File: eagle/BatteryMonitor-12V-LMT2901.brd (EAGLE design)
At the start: 40.6 x 27.9 mm, 20 parts, among them IC1 LMT2901N

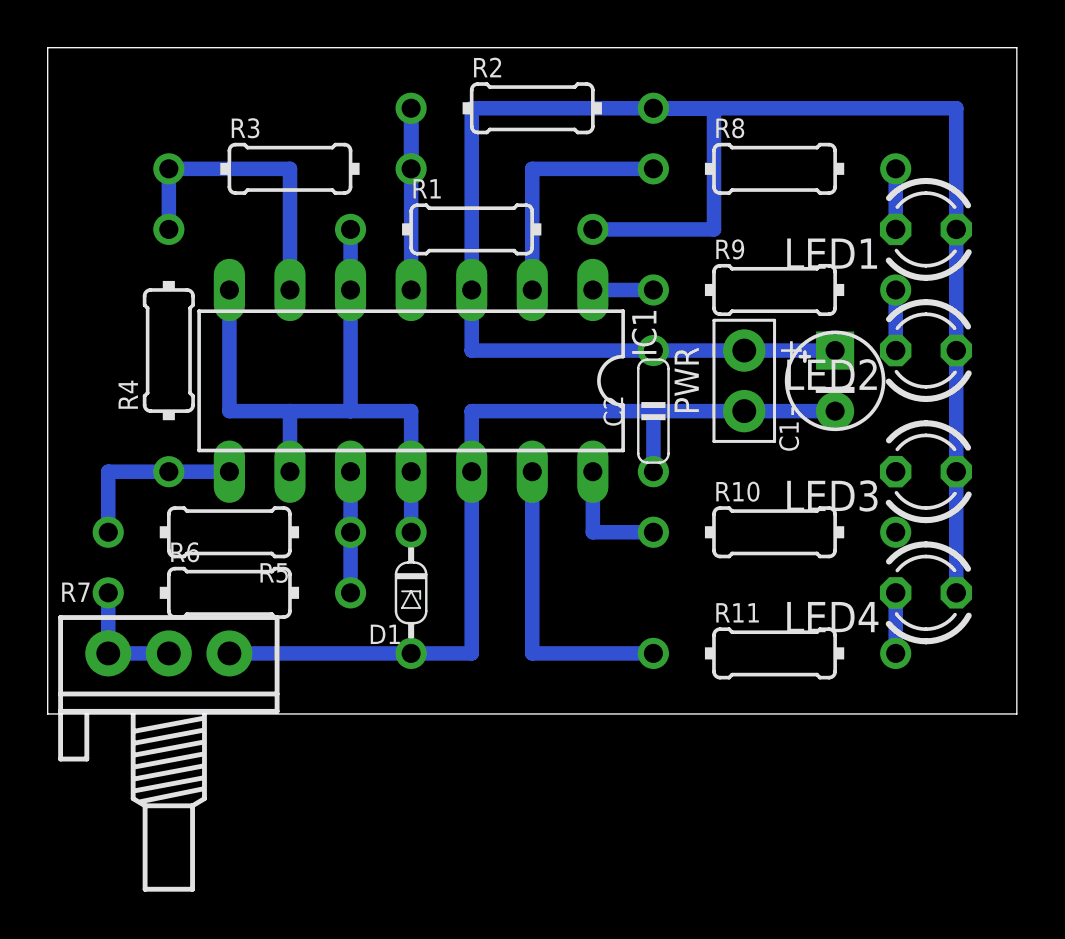
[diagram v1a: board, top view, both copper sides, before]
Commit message: ...
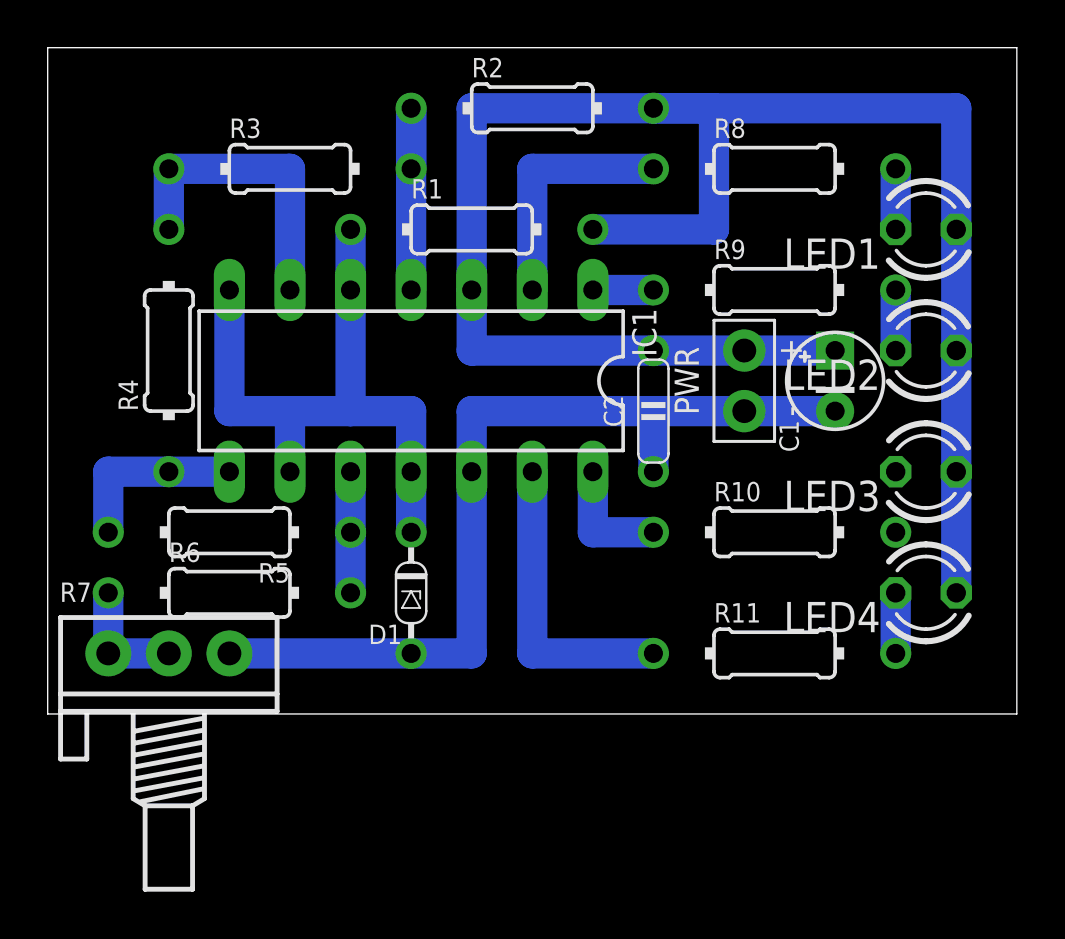
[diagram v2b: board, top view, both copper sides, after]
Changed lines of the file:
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@@
 <contactref element="C1" pad="-"/>
 <contactref element="R7" pad="3"/>
-<wire x1="17.78" y1="11.43" x2="17.78" y2="3.81" width="0.6096" layer="16"/>
-<wire x1="15.24" y1="3.81" x2="7.62" y2="3.81" width="0.6096" layer="16"/>
-<wire x1="25.4" y1="11.43" x2="25.4" y2="13.97" width="0.6096" layer="16"/>
-<wire x1="25.4" y1="13.97" x2="17.78" y2="13.97" width="0.6096" layer="16"/>
-<wire x1="17.78" y1="13.97" x2="17.78" y2="11.43" width="0.6096" layer="16"/>
-<wire x1="15.24" y1="3.81" x2="17.78" y2="3.81" width="0.6096" layer="16"/>
-<wire x1="33.02" y1="13.97" x2="25.4" y2="13.97" width="0.6096" layer="16"/>
+<wire x1="17.78" y1="11.43" x2="17.78" y2="3.81" width="1.27" layer="16"/>
+<wire x1="15.24" y1="3.81" x2="7.62" y2="3.81" width="1.27" layer="16"/>
+<wire x1="25.4" y1="11.43" x2="25.4" y2="13.97" width="1.27" layer="16"/>
+<wire x1="25.4" y1="13.97" x2="17.78" y2="13.97" width="1.27" layer="16"/>
+<wire x1="17.78" y1="13.97" x2="17.78" y2="11.43" width="1.27" layer="16"/>
+<wire x1="15.24" y1="3.81" x2="17.78" y2="3.81" width="1.27" layer="16"/>
+<wire x1="33.02" y1="13.97" x2="25.4" y2="13.97" width="1.27" layer="16"/>
 <wire x1="33.02" y1="13.97" x2="29.21" y2="13.97" width="0" layer="19" extent="1-1"/>
 </signal>
@@
 <contactref element="R11" pad="2"/>
 <contactref element="LED4" pad="K"/>
-<wire x1="35.56" y1="3.81" x2="35.56" y2="6.35" width="0.6096" layer="16"/>
+<wire x1="35.56" y1="3.81" x2="35.56" y2="6.35" width="1.27" layer="16"/>
 </signal>
 <signal name="N$2">
@@
 <contactref element="R9" pad="2"/>
 <contactref element="LED2" pad="K"/>
-<wire x1="35.56" y1="19.05" x2="35.56" y2="16.51" width="0.6096" layer="16"/>
+<wire x1="35.56" y1="19.05" x2="35.56" y2="16.51" width="1.27" layer="16"/>
 </signal>
 <signal name="N$4">
 <contactref element="R8" pad="2"/>
 <contactref element="LED1" pad="K"/>
-<wire x1="35.56" y1="24.13" x2="35.56" y2="21.59" width="0.6096" layer="16"/>
+<wire x1="35.56" y1="24.13" x2="35.56" y2="21.59" width="1.27" layer="16"/>
 </signal>
 <signal name="N$5">
 <contactref element="R8" pad="1"/>
 <contactref element="IC1" pad="2"/>
-<wire x1="25.4" y1="24.13" x2="20.32" y2="24.13" width="0.6096" layer="16"/>
-<wire x1="20.32" y1="24.13" x2="20.32" y2="19.05" width="0.6096" layer="16"/>
+<wire x1="25.4" y1="24.13" x2="20.32" y2="24.13" width="1.27" layer="16"/>
+<wire x1="20.32" y1="24.13" x2="20.32" y2="19.05" width="1.27" layer="16"/>
 </signal>
 <signal name="N$6">
 <contactref element="IC1" pad="1"/>
 <contactref element="R9" pad="1"/>
-<wire x1="25.4" y1="19.05" x2="22.86" y2="19.05" width="0.6096" layer="16"/>
+<wire x1="25.4" y1="19.05" x2="22.86" y2="19.05" width="1.27" layer="16"/>
 </signal>
 <signal name="N$7">
 <contactref element="IC1" pad="14"/>
 <contactref element="R10" pad="1"/>
-<wire x1="25.4" y1="8.89" x2="22.86" y2="8.89" width="0.6096" layer="16"/>
-<wire x1="22.86" y1="8.89" x2="22.86" y2="11.43" width="0.6096" layer="16"/>
+<wire x1="25.4" y1="8.89" x2="22.86" y2="8.89" width="1.27" layer="16"/>
+<wire x1="22.86" y1="8.89" x2="22.86" y2="11.43" width="1.27" layer="16"/>
 </signal>
 <signal name="N$8">
 <contactref element="IC1" pad="13"/>
 <contactref element="R11" pad="1"/>
-<wire x1="20.32" y1="11.43" x2="20.32" y2="3.81" width="0.6096" layer="16"/>
-<wire x1="20.32" y1="3.81" x2="25.4" y2="3.81" width="0.6096" layer="16"/>
+<wire x1="20.32" y1="11.43" x2="20.32" y2="3.81" width="1.27" layer="16"/>
+<wire x1="20.32" y1="3.81" x2="25.4" y2="3.81" width="1.27" layer="16"/>
 </signal>
 <signal name="N$9">
@@
 <contactref element="IC1" pad="9"/>
 <contactref element="IC1" pad="11"/>
-<wire x1="12.7" y1="19.05" x2="12.7" y2="13.97" width="0.6096" layer="16"/>
-<wire x1="15.24" y1="11.43" x2="15.24" y2="13.97" width="0.6096" layer="16"/>
-<wire x1="10.16" y1="13.97" x2="7.62" y2="13.97" width="0.6096" layer="16"/>
-<wire x1="12.7" y1="13.97" x2="10.16" y2="13.97" width="0.6096" layer="16"/>
-<wire x1="10.16" y1="13.97" x2="10.16" y2="11.43" width="0.6096" layer="16"/>
-<wire x1="7.62" y1="19.05" x2="7.62" y2="13.97" width="0.6096" layer="16"/>
-<wire x1="12.7" y1="21.59" x2="12.7" y2="19.05" width="0.6096" layer="16"/>
-<wire x1="12.7" y1="13.97" x2="15.24" y2="13.97" width="0.6096" layer="16"/>
-<wire x1="15.24" y1="11.43" x2="15.24" y2="8.89" width="0.6096" layer="16"/>
+<wire x1="12.7" y1="19.05" x2="12.7" y2="13.97" width="1.27" layer="16"/>
+<wire x1="15.24" y1="11.43" x2="15.24" y2="13.97" width="1.27" layer="16"/>
+<wire x1="10.16" y1="13.97" x2="7.62" y2="13.97" width="1.27" layer="16"/>
+<wire x1="12.7" y1="13.97" x2="10.16" y2="13.97" width="1.27" layer="16"/>
+<wire x1="10.16" y1="13.97" x2="10.16" y2="11.43" width="1.27" layer="16"/>
+<wire x1="7.62" y1="19.05" x2="7.62" y2="13.97" width="1.27" layer="16"/>
+<wire x1="12.7" y1="21.59" x2="12.7" y2="19.05" width="1.27" layer="16"/>
+<wire x1="12.7" y1="13.97" x2="15.24" y2="13.97" width="1.27" layer="16"/>
+<wire x1="15.24" y1="11.43" x2="15.24" y2="8.89" width="1.27" layer="16"/>
 </signal>
 <signal name="N$10">
@@
 <contactref element="R3" pad="2"/>
 <contactref element="IC1" pad="4"/>
-<wire x1="15.24" y1="26.67" x2="15.24" y2="24.13" width="0.6096" layer="16"/>
-<wire x1="15.24" y1="26.67" x2="15.24" y2="19.05" width="0.6096" layer="16"/>
+<wire x1="15.24" y1="26.67" x2="15.24" y2="24.13" width="1.27" layer="16"/>
+<wire x1="15.24" y1="26.67" x2="15.24" y2="19.05" width="1.27" layer="16"/>
 </signal>
 <signal name="N$11">
@@
 <contactref element="R3" pad="1"/>
 <contactref element="R4" pad="2"/>
-<wire x1="10.16" y1="19.05" x2="10.16" y2="24.13" width="0.6096" layer="16"/>
-<wire x1="5.08" y1="21.59" x2="5.08" y2="24.13" width="0.6096" layer="16"/>
-<wire x1="5.08" y1="24.13" x2="10.16" y2="24.13" width="0.6096" layer="16"/>
+<wire x1="10.16" y1="19.05" x2="10.16" y2="24.13" width="1.27" layer="16"/>
+<wire x1="5.08" y1="21.59" x2="5.08" y2="24.13" width="1.27" layer="16"/>
+<wire x1="5.08" y1="24.13" x2="10.16" y2="24.13" width="1.27" layer="16"/>
 </signal>
 <signal name="N$12">
@@
 <contactref element="R4" pad="1"/>
 <contactref element="R5" pad="2"/>
-<wire x1="7.62" y1="11.43" x2="5.08" y2="11.43" width="0.6096" layer="16"/>
-<wire x1="2.54" y1="8.89" x2="2.54" y2="11.43" width="0.6096" layer="16"/>
-<wire x1="2.54" y1="11.43" x2="5.08" y2="11.43" width="0.6096" layer="16"/>
+<wire x1="7.62" y1="11.43" x2="5.08" y2="11.43" width="1.27" layer="16"/>
+<wire x1="2.54" y1="8.89" x2="2.54" y2="11.43" width="1.27" layer="16"/>
+<wire x1="2.54" y1="11.43" x2="5.08" y2="11.43" width="1.27" layer="16"/>
 </signal>
 <signal name="N$13">
@@
 <contactref element="R5" pad="1"/>
 <contactref element="R6" pad="2"/>
-<wire x1="12.7" y1="8.89" x2="12.7" y2="11.43" width="0.6096" layer="16"/>
-<wire x1="12.7" y1="6.35" x2="12.7" y2="8.89" width="0.6096" layer="16"/>
+<wire x1="12.7" y1="8.89" x2="12.7" y2="11.43" width="1.27" layer="16"/>
+<wire x1="12.7" y1="6.35" x2="12.7" y2="8.89" width="1.27" layer="16"/>
 </signal>
 <signal name="VCC">
@@
 <contactref element="LED4" pad="A"/>
 <contactref element="IC1" pad="3"/>
-<wire x1="38.1" y1="6.35" x2="38.1" y2="16.51" width="0.6096" layer="16"/>
-<wire x1="38.1" y1="16.51" x2="38.1" y2="21.59" width="0.6096" layer="16"/>
-<wire x1="17.78" y1="19.05" x2="17.78" y2="26.67" width="0.6096" layer="16"/>
-<wire x1="17.78" y1="26.67" x2="25.4" y2="26.67" width="0.6096" layer="16"/>
-<wire x1="25.4" y1="26.67" x2="38.1" y2="26.67" width="0.6096" layer="16"/>
-<wire x1="38.1" y1="26.67" x2="38.1" y2="21.59" width="0.6096" layer="16"/>
-<wire x1="22.86" y1="21.59" x2="27.94" y2="21.59" width="0.6096" layer="16"/>
-<wire x1="27.94" y1="21.59" x2="27.94" y2="26.67" width="0.6096" layer="16"/>
-<wire x1="27.94" y1="26.67" x2="25.4" y2="26.67" width="0.6096" layer="16"/>
+<wire x1="38.1" y1="6.35" x2="38.1" y2="16.51" width="1.27" layer="16"/>
+<wire x1="38.1" y1="16.51" x2="38.1" y2="21.59" width="1.27" layer="16"/>
+<wire x1="17.78" y1="19.05" x2="17.78" y2="26.67" width="1.27" layer="16"/>
+<wire x1="17.78" y1="26.67" x2="25.4" y2="26.67" width="1.27" layer="16"/>
+<wire x1="25.4" y1="26.67" x2="38.1" y2="26.67" width="1.27" layer="16"/>
+<wire x1="38.1" y1="26.67" x2="38.1" y2="21.59" width="1.27" layer="16"/>
+<wire x1="22.86" y1="21.59" x2="27.94" y2="21.59" width="1.27" layer="16"/>
+<wire x1="27.94" y1="21.59" x2="27.94" y2="26.67" width="1.27" layer="16"/>
+<wire x1="27.94" y1="26.67" x2="25.4" y2="26.67" width="1.27" layer="16"/>
 <contactref element="PWR" pad="2"/>
 <contactref element="C2" pad="1"/>
 <contactref element="C1" pad="+"/>
-<wire x1="25.4" y1="16.51" x2="17.78" y2="16.51" width="0.6096" layer="16"/>
-<wire x1="17.78" y1="16.51" x2="17.78" y2="19.05" width="0.6096" layer="16"/>
-<wire x1="33.02" y1="16.51" x2="25.4" y2="16.51" width="0.6096" layer="16"/>
+<wire x1="25.4" y1="16.51" x2="17.78" y2="16.51" width="1.27" layer="16"/>
+<wire x1="17.78" y1="16.51" x2="17.78" y2="19.05" width="1.27" layer="16"/>
+<wire x1="33.02" y1="16.51" x2="25.4" y2="16.51" width="1.27" layer="16"/>
 <wire x1="38.1" y1="16.51" x2="38.1" y2="12.7" width="0" layer="19" extent="1-16"/>
 <wire x1="38.1" y1="12.7" x2="38.1" y2="11.43" width="0" layer="19" extent="16-16"/>
@@
 <contactref element="R7" pad="2"/>
 <contactref element="R7" pad="1"/>
-<wire x1="5.08" y1="3.81" x2="2.54" y2="3.81" width="0.6096" layer="16"/>
+<wire x1="5.08" y1="3.81" x2="2.54" y2="3.81" width="1.27" layer="16"/>
 <contactref element="R6" pad="1"/>
-<wire x1="2.54" y1="3.81" x2="2.54" y2="6.35" width="0.6096" layer="16"/>
+<wire x1="2.54" y1="3.81" x2="2.54" y2="6.35" width="1.27" layer="16"/>
 </signal>
 </signals>
